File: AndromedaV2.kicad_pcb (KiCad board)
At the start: 2 copper layers, 100 x 65 mm, 94 parts, among them J1 USB_MINIB, J10 TEST_1P, J11 TEST_1P, J12 Micro_SD_Card, J13 TEST_1P, J14 TEST_1P, J15 TEST_1P, J16 TEST_1P, J17 TEST_1P, J18 GPS, J19 Radio, J2 TEST_1P, J20 Recovery, J21 Propulsion, J22 Tank Pressure, J23 Low Pressure, J24 Conn_01x06, J25 Battery, J26 Launch Systems, J27 SD, J3 TEST_1P, J4 TEST_1P, J5 TEST_1P, J6 TEST_1P, J7 TEST_1P, J8 TEST_1P, J9 TEST_1P, U1 FT230XS, U2 TPS562200, U3 AP2210-3.3, U4 AP2204K-5.0, U5 STM32F405R, U6 MS5607, U7 LSM9DS1, Y1 Crystal_8MHz_18pf

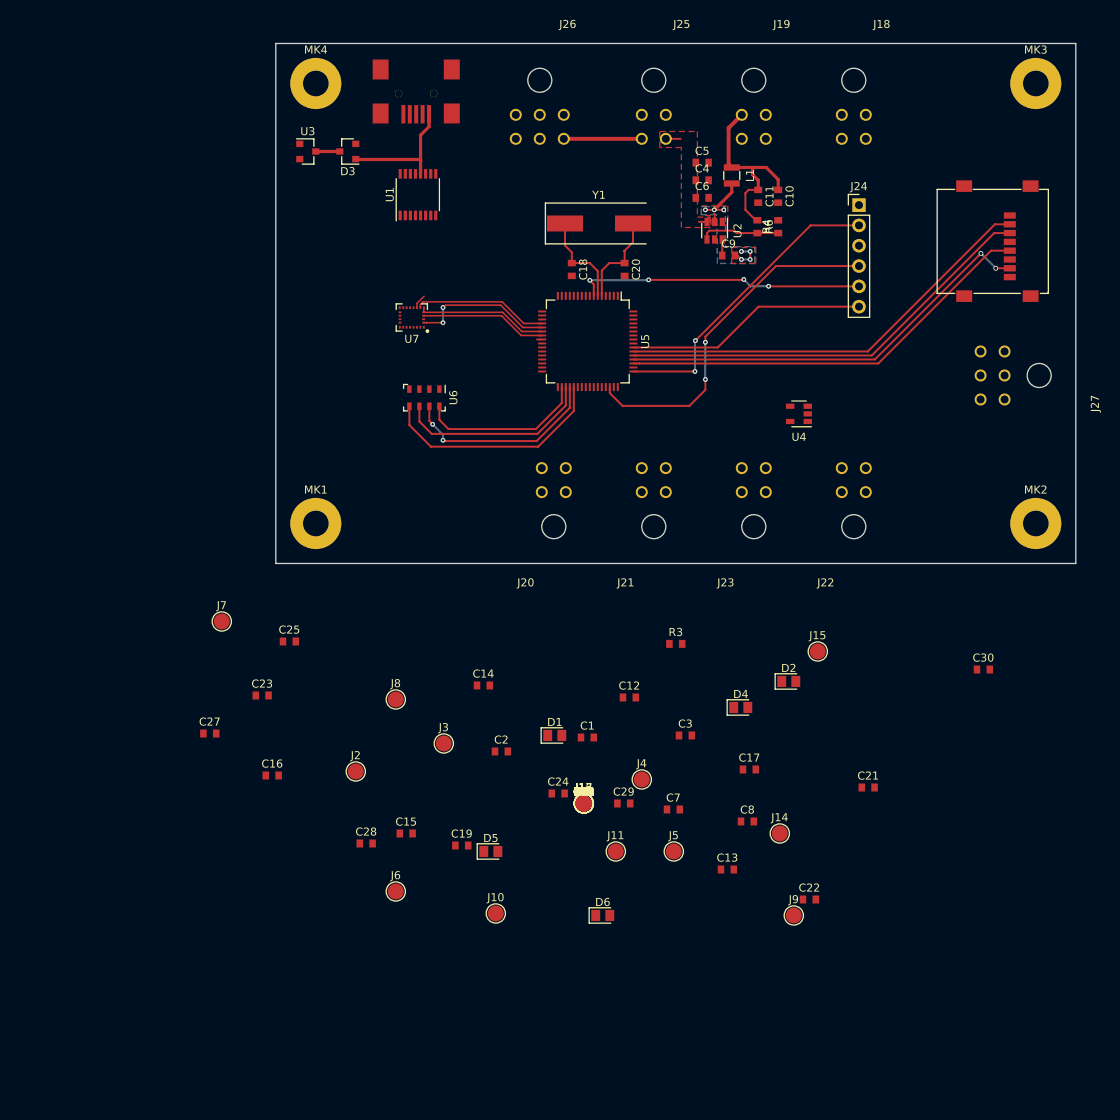
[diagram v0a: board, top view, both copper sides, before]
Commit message: further work on schematic and PCB
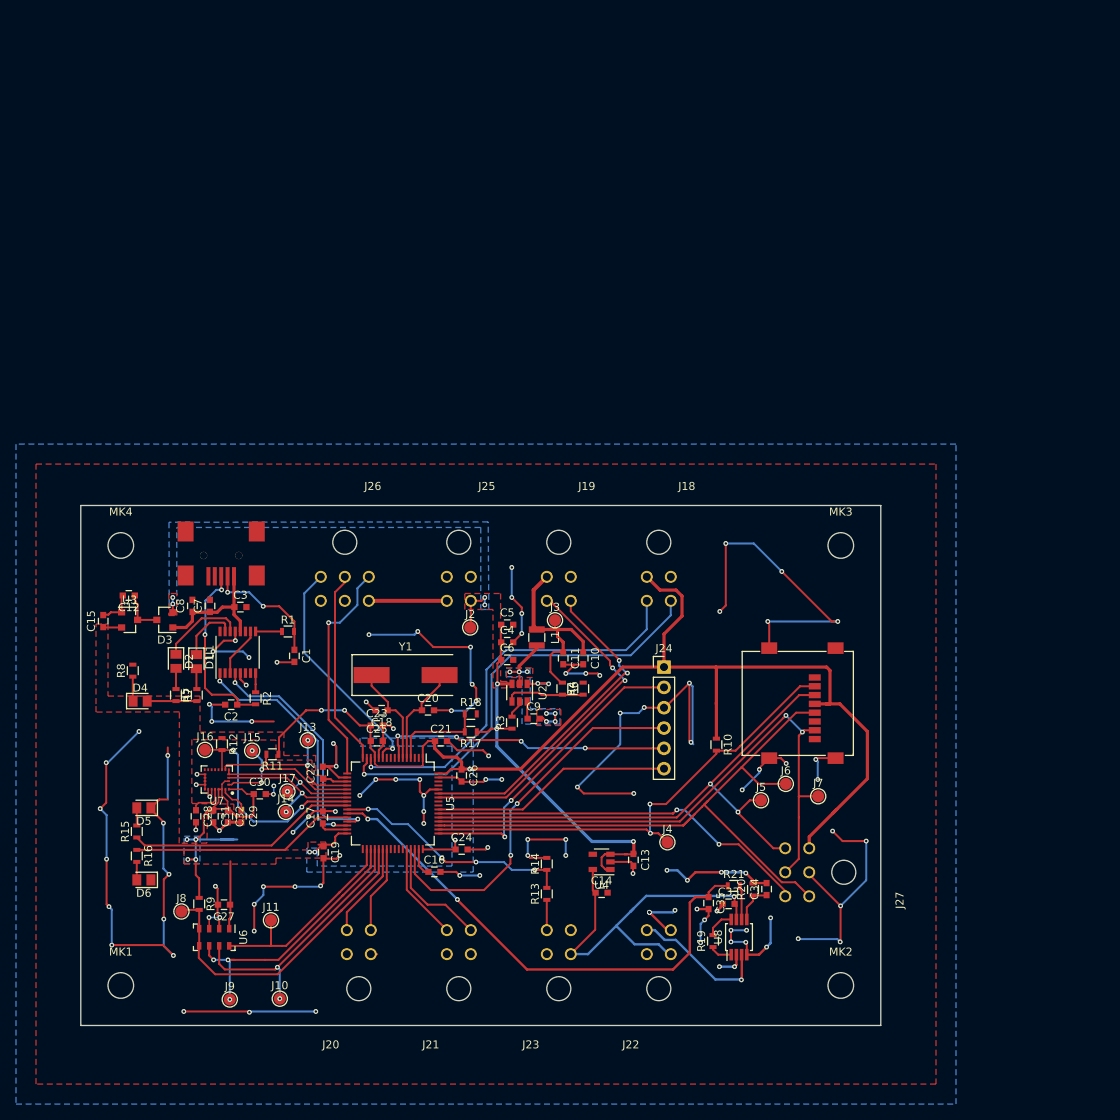
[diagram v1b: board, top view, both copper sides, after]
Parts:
- removed JP1, JP2: Jumper_NC_Small, Resistor_SMD:R_0603_1608Metric
- added C33: 0.1uF, Capacitors_SMD:C_0603, F.Cu at (166.6, 117.5)
- added C34: 0.5nF, Capacitors_SMD:C_0603, F.Cu at (171.3, 115.7)
- added C35: 1uF, Capacitors_SMD:C_0603, F.Cu at (164.1, 117.5)
- added R15: 330, Resistors_SMD:R_0603, F.Cu at (92.6, 108.5)
- added R16: 330, Resistors_SMD:R_0603, F.Cu at (92.6, 111.5)
- added R17: 30K, Resistors_SMD:R_0603, F.Cu at (134.4, 96.0)
- added R18: 10K, Resistors_SMD:R_0603, F.Cu at (134.4, 93.8)
- added R19: 13K, Resistors_SMD:R_0603, F.Cu at (164.7, 122.2)
- added R20: 200K, Resistors_SMD:R_0603, F.Cu at (169.7, 115.8)
- added R21: 100, Resistors_SMD:R_0603, F.Cu at (167.2, 115.3)
- added U8: INA326, Housings_SSOP:MSOP-8_3x3mm_Pitch0.65mm, F.Cu at (167.9, 121.7)
- C1, C10, C11, C12, C13, C14, C15, C16, C17, C18, C19, C2, C20, C21, C22, C23, C24, C25, C26, C27, C28, C29, C3, C30, C31, C32, C4, C5, C6, C7, C8, C9: footprint Capacitor_SMD:C_0603_1608Metric -> Capacitors_SMD:C_0603
- J10, J11, J13, J14, J15, J16, J17, J2, J3, J4, J5, J6, J7, J8, J9: footprint TestPoint:TestPoint_Pad_D2.0mm -> Connectors_TestPoints:Test_Point_Pad_d1.5mm
- MK1, MK2, MK3, MK4: value Mounting_Hole_PAD -> Mounting_Hole; footprint MountingHole:MountingHole_3.2mm_M3_Pad -> Mounting_Holes:MountingHole_3.2mm_M3
- R1, R10, R11, R12, R2, R3, R4, R5, R6, R7, R8, R9: footprint Resistor_SMD:R_0603_1608Metric -> Resistors_SMD:R_0603
- R13: value 330 -> 100K; footprint Resistor_SMD:R_0603_1608Metric -> Resistors_SMD:R_0603
- R14: value 330 -> 133K; footprint Resistor_SMD:R_0603_1608Metric -> Resistors_SMD:R_0603
- moved C30 91.8 mm to (108.0, 103.8)
- moved J7 77.7 mm to (177.8, 104.1)
- moved D2 76.6 mm to (97.5, 87.2), turned to 270 degrees
- moved D4 75.1 mm to (93.0, 92.2)
- moved C8 74.4 mm to (99.6, 80.3), turned to 90 degrees
- moved U6 72.4 mm to (102.3, 121.7)
- moved J15 71.8 mm to (107.0, 98.4)
- moved J9 71.3 mm to (104.2, 129.5)
- moved J27 66.7 mm to (185.6, 113.6)
- moved C12 63.9 mm to (91.6, 79.0), turned to 180 degrees
- moved C7 63.3 mm to (101.8, 80.3), turned to 90 degrees
- moved D3 62.9 mm to (96.1, 82.0)
- moved C22 62.9 mm to (115.9, 101.2), turned to 90 degrees
- moved C9 62.8 mm to (142.2, 94.4)
- moved C5 62.7 mm to (138.9, 82.7)
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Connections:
- net Baro_~CS renamed BARO_~CS
- J12 pad 2: SD_~CS -> SD1_~CS
- J13 pad 1: Net-(J13-Pad1) -> A/G_~CS
- J14 pad 1: Net-(J14-Pad1) -> SPI1_MOSI
- J15 pad 1: Net-(J15-Pad1) -> SPI1_SCK
- J18 pad 2: Net-(J18-Pad2) -> GND
- J18 pad 3: Net-(J18-Pad3) -> UART4_TX
- J18 pad 4: Net-(J18-Pad4) -> UART4_RX
- J19 pad 2: Net-(J19-Pad2) -> GND
- J19 pad 3: Net-(J19-Pad3) -> UART1_TX
- J19 pad 4: Net-(J19-Pad4) -> UART1_RX
- J20 pad 1: Net-(J20-Pad1) -> GND
- J20 pad 2: Net-(J20-Pad2) -> GND
- J20 pad 3: Net-(J20-Pad3) -> RECOVERY_2
- J20 pad 4: Net-(J20-Pad4) -> RECOVERY_1
- J21 pad 1: Net-(J21-Pad1) -> GND
- J21 pad 2: Net-(J21-Pad2) -> GND
- J21 pad 3: Net-(J21-Pad3) -> PROPULSION2
- J21 pad 4: Net-(J21-Pad4) -> PROPULSION1
- J22 pad 1: Net-(J22-Pad1) -> +5V
- J22 pad 2: Net-(J22-Pad2) -> GND
- J22 pad 3: Net-(J22-Pad3) -> GND
- J23 pad 2: Net-(J23-Pad2) -> GND
- J23 pad 3: Net-(J23-Pad3) -> GND
- J26 pad 1: Net-(J26-Pad1) -> LAUNCH
- J26 pad 2: Net-(J26-Pad2) -> UART2_TX
- J26 pad 3: Net-(J26-Pad3) -> UART2_RX
- J26 pad 5: Net-(J26-Pad5) -> GND
- J27 pad 1: Net-(J27-Pad1) -> +3V3
- J27 pad 2: Net-(J27-Pad2) -> GND
- J27 pad 3: Net-(J27-Pad3) -> SPI3_SCK
- J27 pad 4: Net-(J27-Pad4) -> SPI3_MOSI
- J27 pad 5: Net-(J27-Pad5) -> SPI3_MISO
- J27 pad 6: Net-(J27-Pad6) -> SD2_~CS
- J4 pad 1: SD_~CS -> SD1_~CS
- MK1 pad 1: GND -> (no net)
- MK2 pad 1: GND -> (no net)
- MK3 pad 1: GND -> (no net)
- MK4 pad 1: GND -> (no net)
- R10 pad 2: SD_~CS -> SD1_~CS
- R13 pad 1: LED1 -> Net-(J23-Pad4)
- R13 pad 2: Net-(D5-Pad2) -> ADC1
- R14 pad 1: LED2 -> ADC1
- R14 pad 2: Net-(D6-Pad2) -> GND
- U1 pad 1: Net-(JP1-Pad1) -> UART3_RX
- U1 pad 4: Net-(JP2-Pad1) -> UART3_TX
- U2 pad 5: Net-(U2-Pad5) -> Net-(R3-Pad2)
- U5 pad 11: Net-(U5-Pad11) -> LAUNCH
- U5 pad 14: Net-(U5-Pad14) -> UART4_TX
- U5 pad 15: Net-(U5-Pad15) -> UART4_RX
- U5 pad 16: Net-(U5-Pad16) -> UART2_TX
- U5 pad 17: MAG_~CS -> UART2_RX
- U5 pad 24: Net-(U5-Pad24) -> MAG_~CS
- U5 pad 25: Net-(U5-Pad25) -> LED1
- U5 pad 26: Net-(U5-Pad26) -> ADC1
- U5 pad 27: Net-(U5-Pad27) -> ADC2
- U5 pad 28: Net-(U5-Pad28) -> LED2
- U5 pad 29: Net-(U5-Pad29) -> UART3_TX
- U5 pad 30: Net-(U5-Pad30) -> UART3_RX
- U5 pad 38: Net-(U5-Pad38) -> RECOVERY_1
- U5 pad 39: Net-(U5-Pad39) -> RECOVERY_2
- U5 pad 44: Net-(U5-Pad44) -> PROPULSION1
- U5 pad 45: Net-(U5-Pad45) -> PROPULSION2
- U5 pad 50: Net-(U5-Pad50) -> SD1_~CS
- U5 pad 54: SD_~CS -> SD2_~CS
- U5 pad 58: Net-(U5-Pad58) -> UART1_TX
- U5 pad 59: Net-(U5-Pad59) -> UART1_RX
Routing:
- net GND: track 0.06 -> 435.7 mm, vias 0 -> 114
- net +3V3: track 0.00 -> 220.8 mm, vias 0 -> 10
- net ADC2: track 0.00 -> 64.1 mm, vias 0 -> 2
- net SD1_~CS: track 0.00 -> 60.2 mm, vias 0 -> 2
- net +BATT: track 2.87 -> 60.6 mm, vias 0 -> 7
- net UART4_RX: track 0.00 -> 54.6 mm, vias 0 -> 1
- net SD_~CS: track 53.6 -> 0.00 mm
- net UART4_TX: track 0.00 -> 50.4 mm, vias 0 -> 1
- net SD2_~CS: track 0.00 -> 48.4 mm, vias 0 -> 2
- net +5V: track 0.00 -> 47.6 mm, vias 0 -> 1
- net UART1_TX: track 0.00 -> 43.6 mm, vias 0 -> 2
- net UART1_RX: track 0.00 -> 41.9 mm, vias 0 -> 2
- net UART3_TX: track 0.00 -> 30.5 mm, vias 0 -> 2
- net ADC1: track 0.00 -> 30.4 mm, vias 0 -> 4
- net UART3_RX: track 0.00 -> 30.0 mm, vias 0 -> 2
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- added copper zone on B.Cu, net +3V3
- added copper zone on F.Cu, net +3V3
- added copper zone on B.Cu, net +BATT
- added copper zone on B.Cu, net GND
- added copper zone on F.Cu, net GND
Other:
- net class Default: clearance 0.2 -> 0.15
- rule trace_clearance: 0.2 -> 0.15
- rule trace_min: 0.2 -> 0.18
